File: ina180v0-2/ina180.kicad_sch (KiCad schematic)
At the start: 6 parts, among them U1 INA180A2

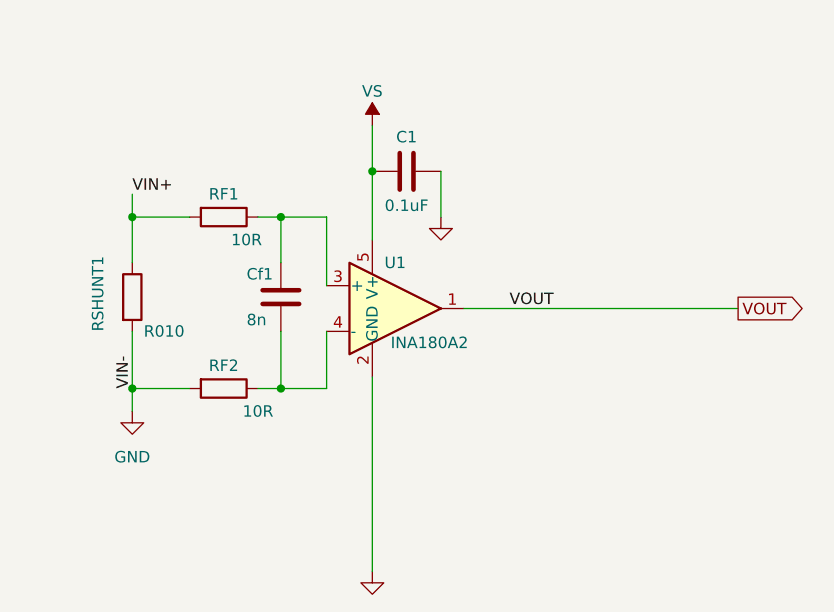
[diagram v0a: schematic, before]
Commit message: Improved schematic
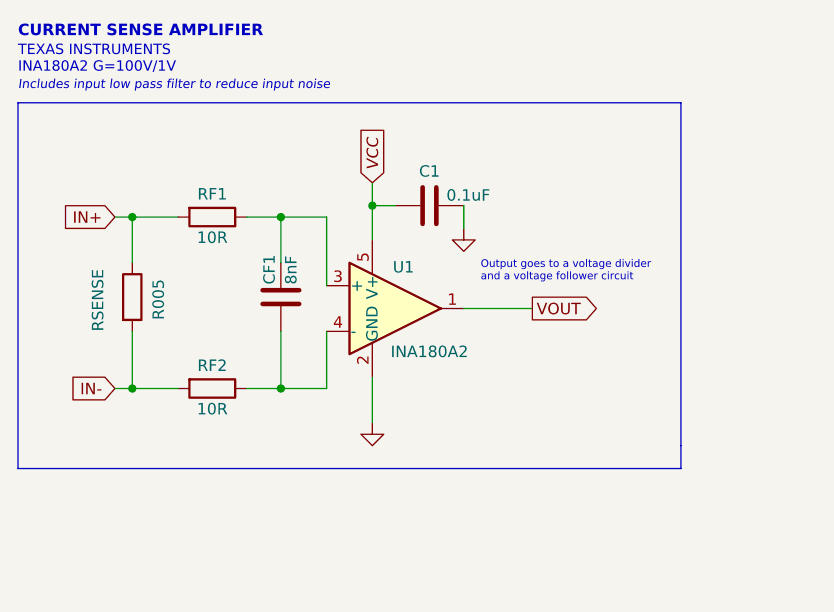
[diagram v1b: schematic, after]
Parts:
- CF1: renamed from Cf1; value 8n -> 8nF
- RSENSE: renamed from RSHUNT1; value R010 -> R005
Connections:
- net GND: no longer RF2.2, RSENSE.2
- net VIN+ renamed IN+
- net VS renamed VCC
- new net IN-: RF2.2, RSENSE.2
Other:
- note added: "CURRENT SENSE AMPLIFIER"
- note added: "Includes input low pass filter to reduce input noise"
- note added: "Output goes to a voltage divider and a voltage follower circuit"
- note added: "TEXAS INSTRUMENTS INA180A2 G=100V/1V"
- moved on the sheet: C1, RF1, RF2
